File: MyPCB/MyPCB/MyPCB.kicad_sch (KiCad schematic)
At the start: 8 parts, among them J1 OLED_DISPLAY, SW1 SW_Push, SW2 SW_Push, SW3 SW_Push, SW4 SW_Push, U1 XIAO-RP2040-DIP

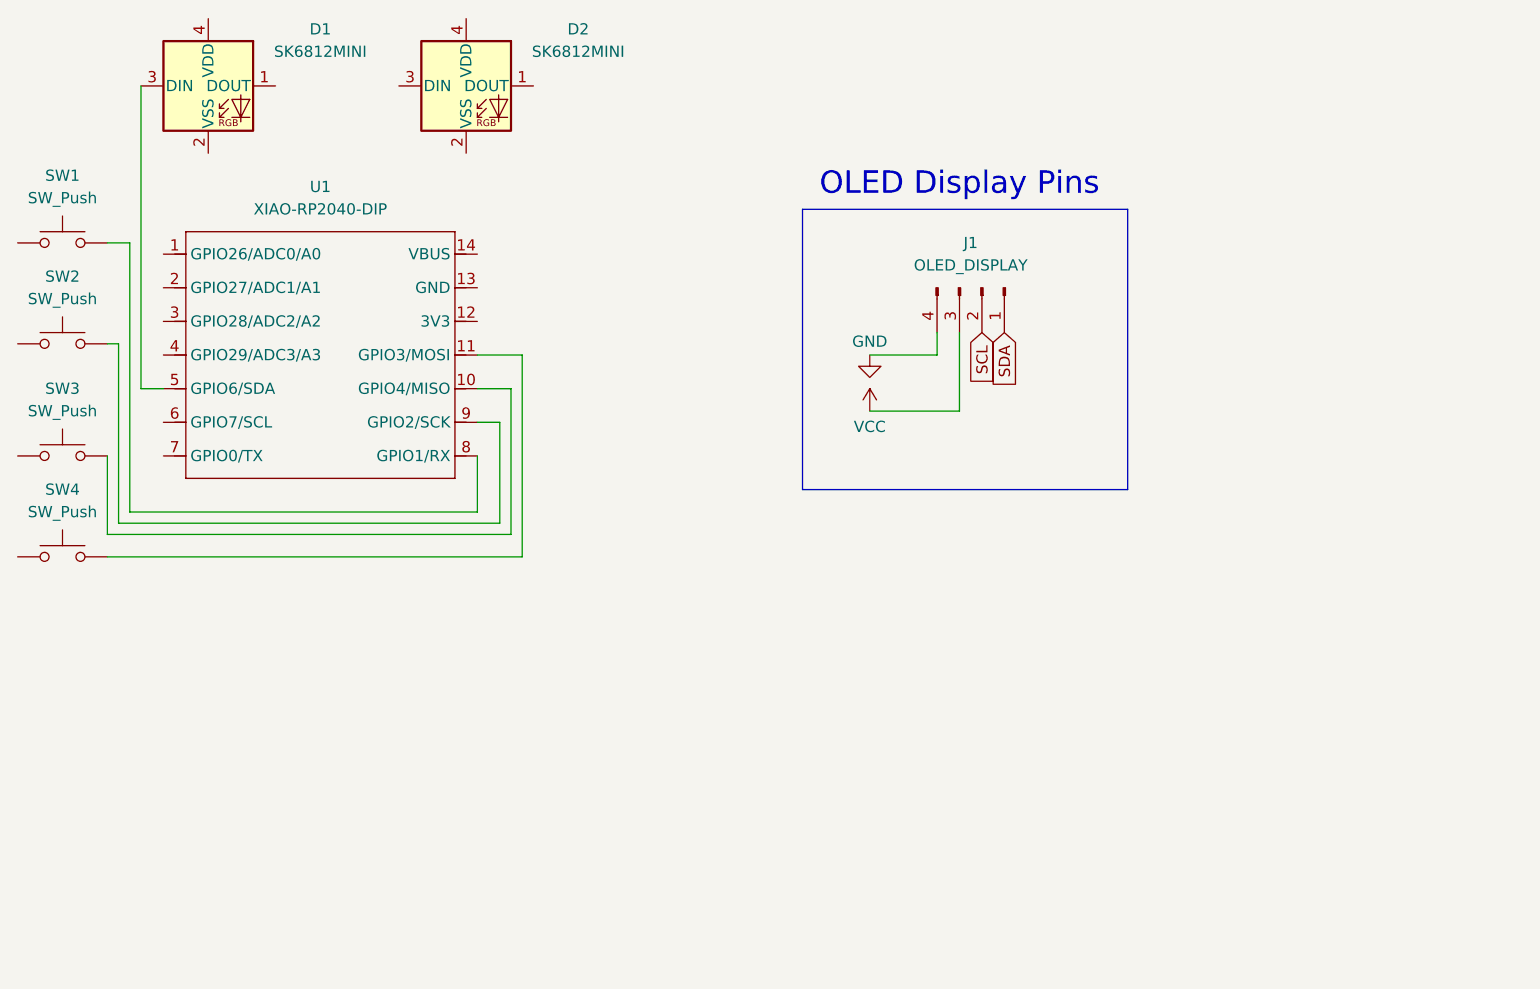
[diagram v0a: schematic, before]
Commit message: Update PCB Design
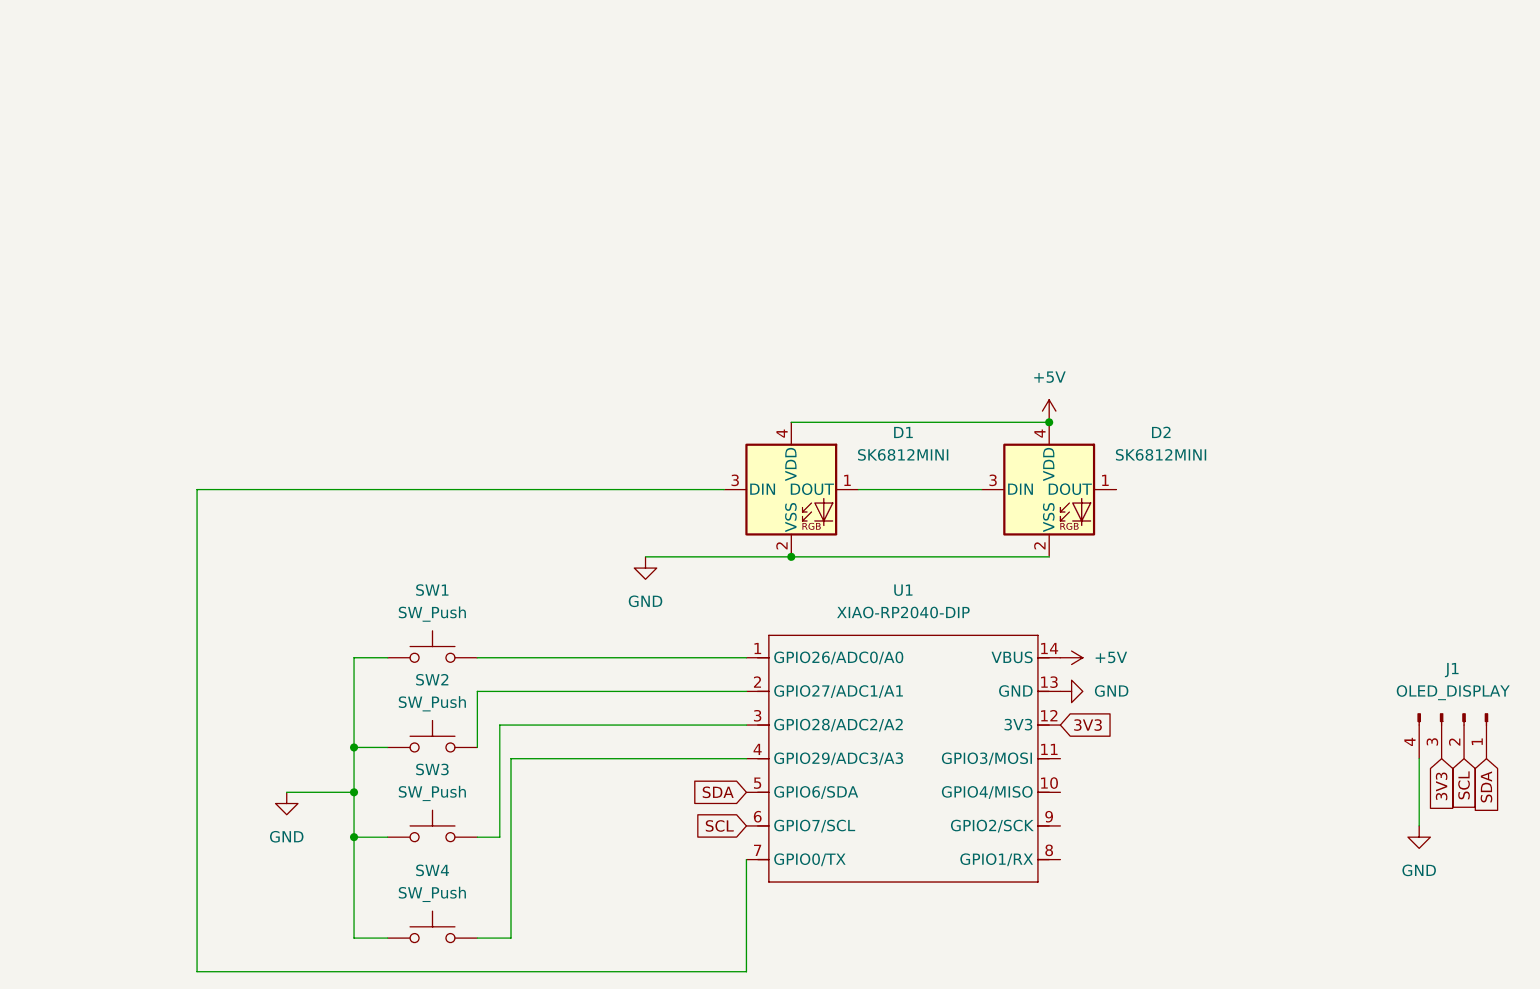
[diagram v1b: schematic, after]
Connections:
- net VCC is gone; now on net 3V3: J1.3 (Pin_3)
- net GND: now also D1.2 (VSS), D2.2 (VSS), SW1.1, SW2.1, SW3.1, SW4.1, U1.13 (GND)
- net SCL: now also U1.6 (GPIO7/SCL)
- net SDA: now also U1.5 (GPIO6/SDA)
- net at SW2.2: now also U1.2 (GPIO27/ADC1/A1); no longer U1.9 (GPIO2/SCK)
- net at U1.1 (GPIO26/ADC0/A0): now also SW1.2
- net at U1.10 (GPIO4/MISO): no longer SW3.2
- net at U1.11 (GPIO3/MOSI): no longer SW4.2
- net 3V3: now reaches U1.12 (3V3)
- net +5V: now reaches U1.14 (VBUS)
- net +5V: now also D1.4 (VDD), D2.4 (VDD)
- net at U1.3 (GPIO28/ADC2/A2): now also SW3.2
- net at U1.4 (GPIO29/ADC3/A3): now also SW4.2
- net at D1.3 (DIN): now also U1.7 (GPIO0/TX); no longer U1.5 (GPIO6/SDA)
- net at U1.8 (GPIO1/RX): no longer SW1.2
- net at D1.1 (DOUT): now also D2.3 (DIN)
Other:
- note removed: "OLED Display Pins"
- company: (none) -> HackClub
- title: (none) -> Arjun's Multi Camera Livestream MacroPad
- moved on the sheet: D1, D2, J1, SW1, SW2, SW3, SW4, U1
